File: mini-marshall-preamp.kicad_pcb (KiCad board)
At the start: 2 copper layers, 134 x 77 mm, 46 parts, among them J1 LO, J2 HI, J3 OUT, J4 6V3, J5 370V GND, J6 370V, J7 6V3 GND, J8 6V3, J9 6V3 GND, U1 6N2P, U2 6N2P

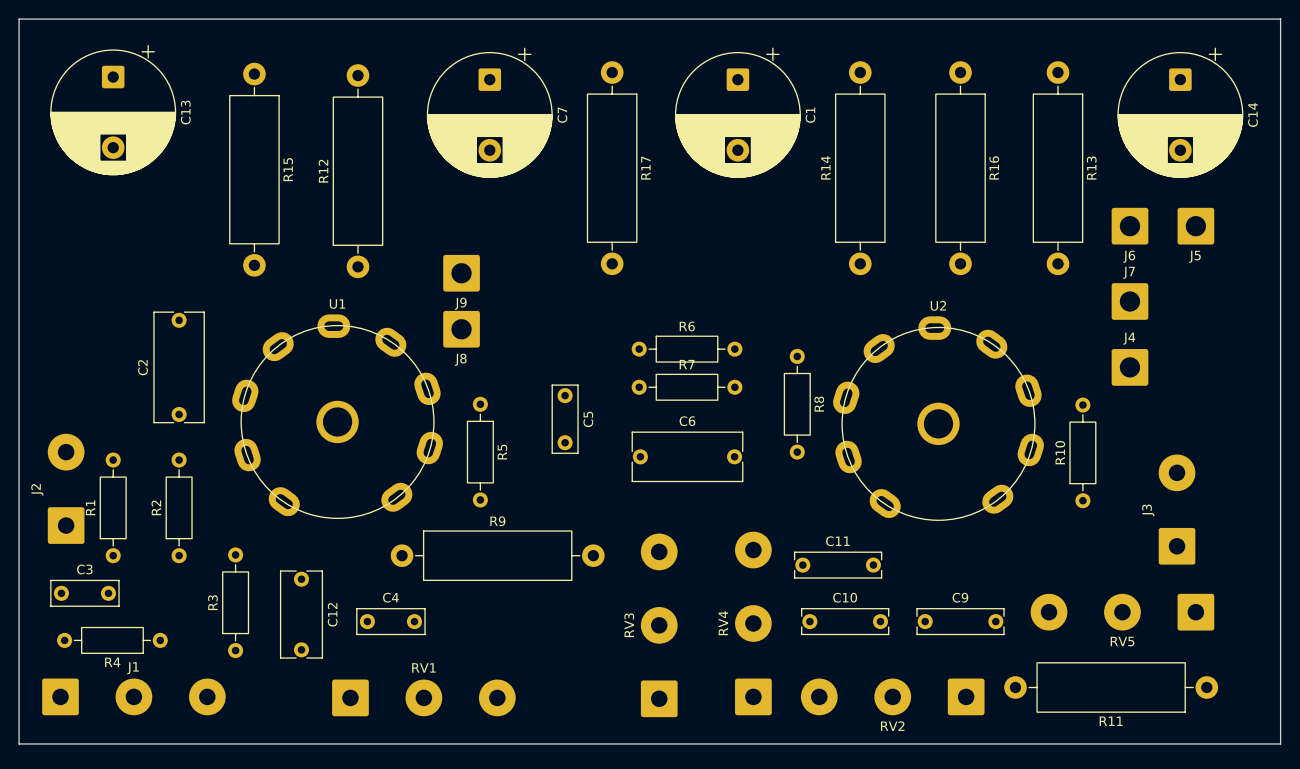
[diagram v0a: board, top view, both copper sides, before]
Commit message: Nice layout
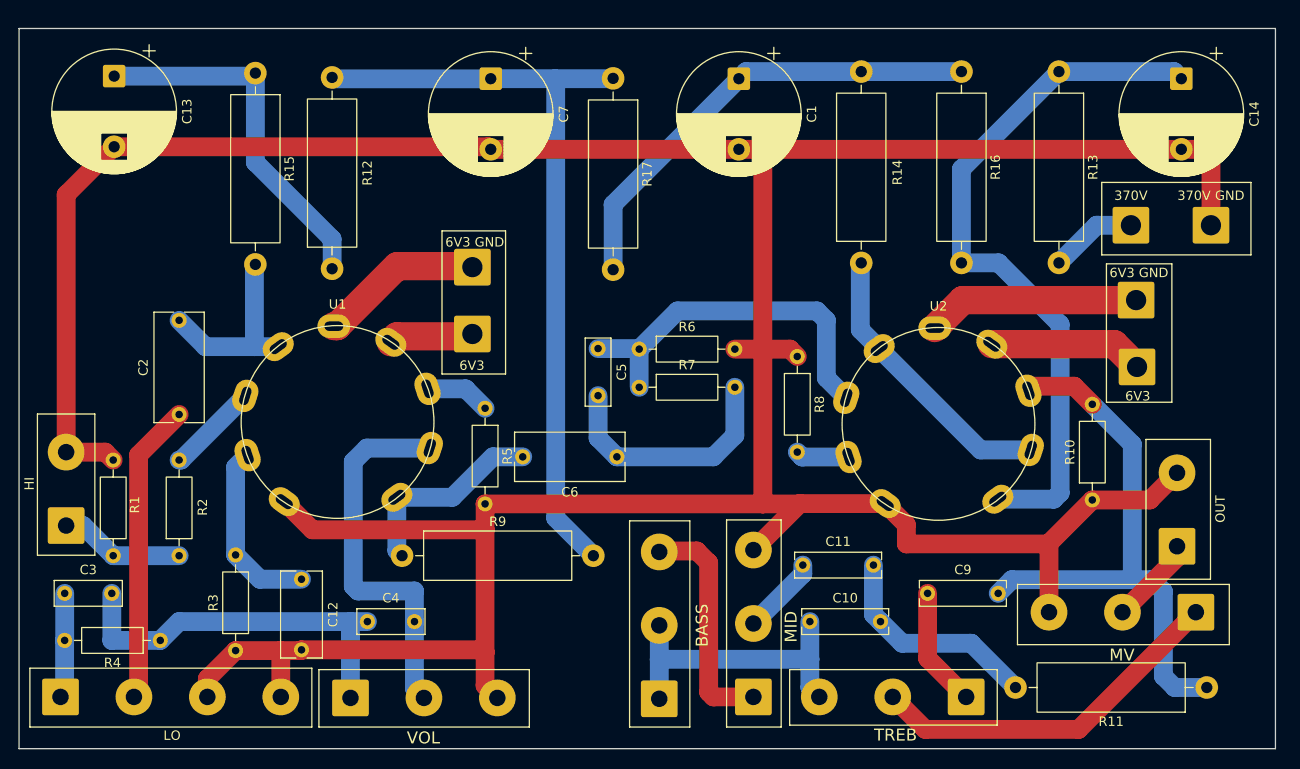
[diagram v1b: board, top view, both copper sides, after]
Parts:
- J1: footprint Connector_Wire:SolderWire-1sqmm_1x03_P7.8mm_D1.4mm_OD3.9mm -> Connector_Wire:SolderWire-1sqmm_1x04_P7.8mm_D1.4mm_OD3.9mm
- moved C5 6.10 mm to (114.5, 84.0)
- moved C9 3.01 mm to (149.5, 110.0)
- moved R12 2.76 mm to (86.2, 75.5)
- moved C6 2.50 mm to (116.5, 95.5), turned to 180 degrees
- moved J5 1.60 mm to (179.6, 70.9)
- moved J9 1.32 mm to (101.2, 75.3)
- moved J8 1.25 mm to (101.2, 82.5)
- moved R10 1.00 mm to (167.0, 100.1)
- moved J4 0.75 mm to (171.8, 86.0)
- moved J7 0.67 mm to (171.7, 78.8)
- moved R5 0.65 mm to (102.5, 90.3)
- moved R17 0.63 mm to (116.1, 55.3)
- moved C3 0.35 mm to (57.9, 110.0)
- moved C1 0.14 mm to (129.5, 55.3)
- moved C14 0.14 mm to (176.5, 55.3)
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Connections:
- net Net-(U2B-A) renamed /anode
- J4 pad 1: /heater -> Net-(J4-Pin_1)
- J8 pad 1: /heater -> Net-(J8-Pin_1)
- U1 pad 4: /heater -> Net-(J8-Pin_1)
- U2 pad 4: /heater -> Net-(J4-Pin_1)
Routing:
- net GND: track 0.00 -> 384.2 mm
- net Net-(C7-Pad1): track 0.00 -> 82.3 mm
- net /anode: track 0.00 -> 75.9 mm
- net Net-(U2B-K): track 0.00 -> 60.9 mm
- net Net-(C1-Pad1): track 0.00 -> 49.8 mm
- net Net-(C3-Pad2): track 0.00 -> 41.1 mm
- net Net-(U1B-G): track 0.00 -> 40.5 mm
- net GND1: track 0.00 -> 40.0 mm
- net Net-(U2A-G): track 0.00 -> 39.5 mm
- net Net-(C13-Pad1): track 0.00 -> 39.3 mm
- net Net-(RV2-Pad2): track 0.00 -> 38.8 mm
- net Net-(C10-Pad1): track 0.00 -> 32.2 mm
- net Net-(J1-SN): track 0.00 -> 32.0 mm
- net Net-(U2A-A): track 0.00 -> 30.5 mm
- net Net-(C5-Pad2): track 0.00 -> 25.9 mm
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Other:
- board size 134 x 77 mm -> 133.4 x 76.5 mm
